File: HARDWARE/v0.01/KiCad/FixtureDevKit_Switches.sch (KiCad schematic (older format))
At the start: 58 parts, among them J10 LED_4, J11 SW_5, J12 LED_5, J13 SW_6, J14 LED_6, J15 SW_7, J2 LED_0, J3 SW_0, J4 SW_1, J5 LED_1, J6 SW_2, J7 LED_3, J8 SW_3, J9 SW_4, SW1 SW_Push_Dual, SW2 SW_Push_Dual, SW3 SW_Push_Dual, SW4 SW_Push_Dual, SW5 SW_Push_Dual, SW6 SW_Push_Dual, SW7 SW_Push_Dual, SW8 SW_Push_Dual

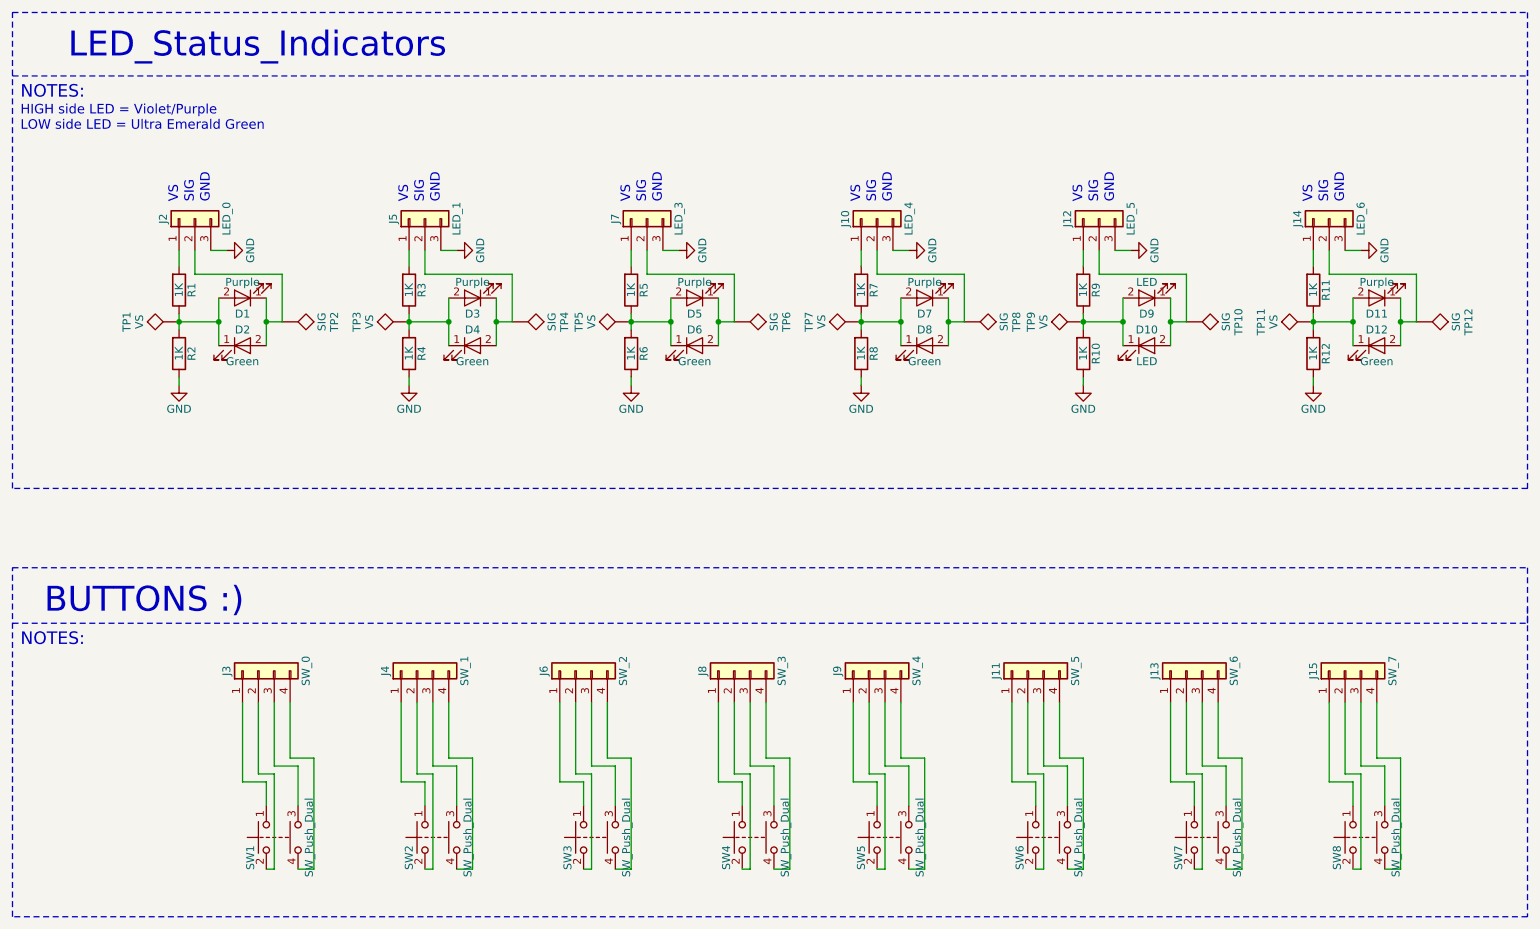
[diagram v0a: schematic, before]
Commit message: beginning pcb layout
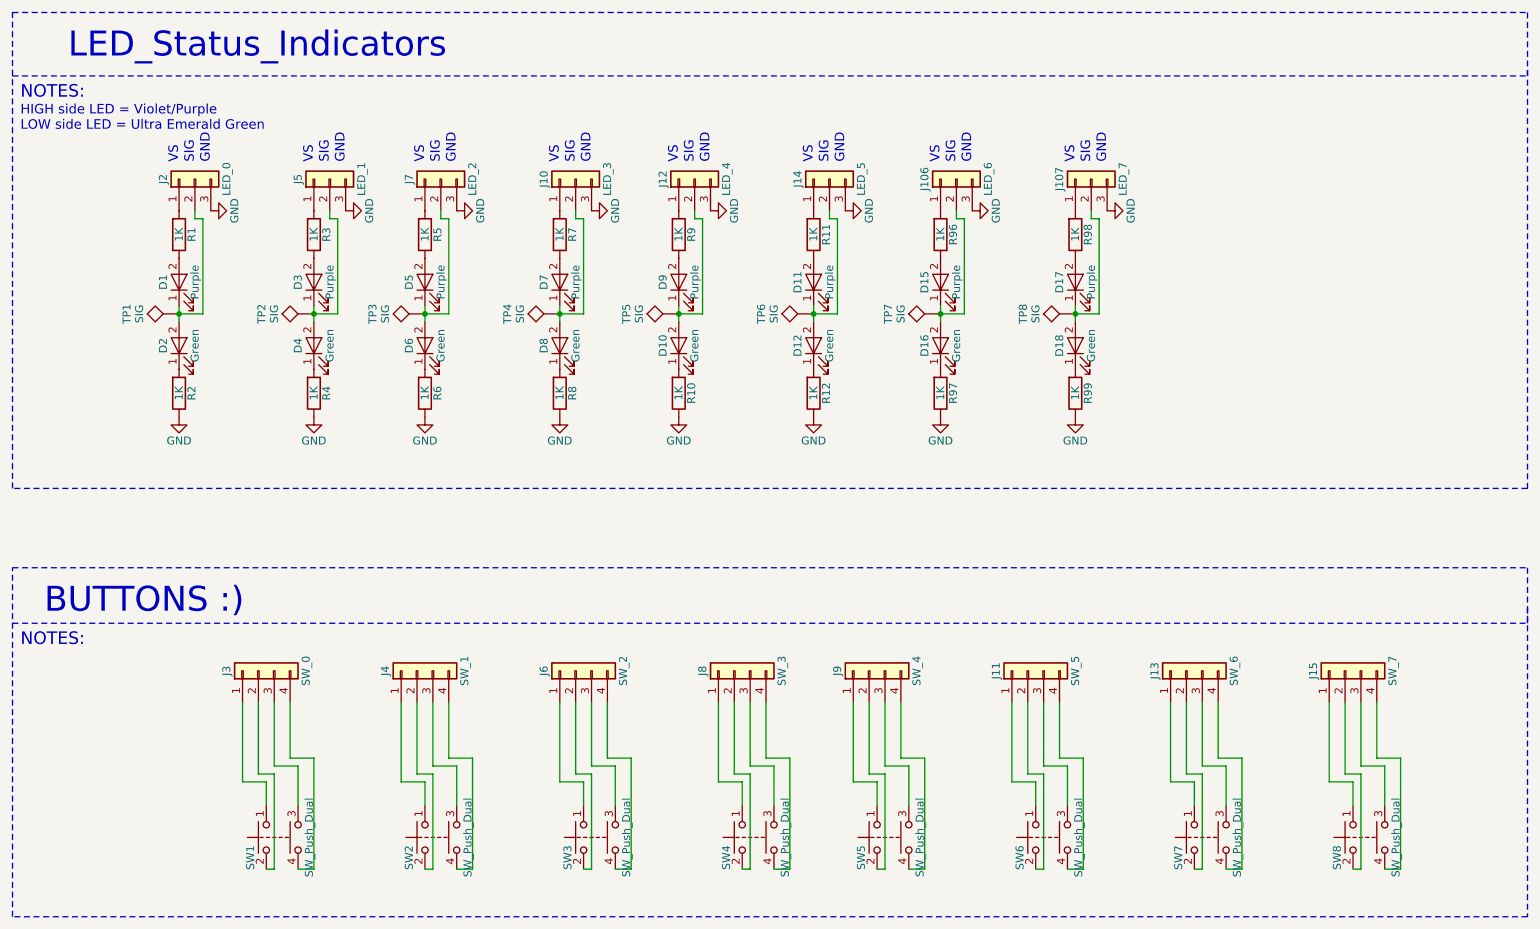
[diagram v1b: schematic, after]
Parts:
- removed TP1, TP11, TP9: VS, TestPoint:TestPoint, symbol TEST
- removed TP10, TP12: SIG, TestPoint:TestPoint, symbol TEST
- added D15, D17: Purple, LEDs:LED_0805_HandSoldering, symbol LED
- added D16, D18: Green, LEDs:LED_0805_HandSoldering, symbol LED
- added J106: LED_6, Pin_Headers:Pin_Header_Straight_1x03_Pitch2.54mm, symbol Conn_01x03
- added J107: LED_7, Pin_Headers:Pin_Header_Straight_1x03_Pitch2.54mm, symbol Conn_01x03
- added R96, R97, R98, R99: 1K, Resistors_SMD:R_0805_HandSoldering, symbol R
- added TP2: SIG, TestPoint:TestPoint, symbol TEST
- D10: value LED -> Green
- D9: value LED -> Purple
- J10: value LED_4 -> LED_3
- J12: value LED_5 -> LED_4
- J14: value LED_6 -> LED_5
- J7: value LED_3 -> LED_2
- TP3, TP5, TP7: value VS -> SIG
- renumbered TP2 to TP1
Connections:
- net GND: now also J106.3 (Pin_3), J107.3 (Pin_3), R97.1, R99.1
- net at D2.1 (K), R2.2: no longer D1.2 (A), R1.1
- net at D3.1 (K), D4.2 (A), J5.2 (Pin_2): now also TP2.1; no longer TP4.1
- net at D5.1 (K), D6.2 (A), J7.2 (Pin_2): now also TP3.1; no longer TP6.1
- net at D7.1 (K), D8.2 (A), J10.2 (Pin_2): now also TP4.1; no longer TP8.1
- net at D10.2 (A), D9.1 (K), J12.2 (Pin_2): now also TP5.1
- net at D10.1 (K), R10.2: no longer D9.2 (A), R9.1
- net at D11.1 (K), D12.2 (A), J14.2 (Pin_2): now also TP6.1
- net at D12.1 (K), R12.2: no longer D11.2 (A), R11.1
- new net: D1.2 (A), R1.1
- new net: D4.1 (K), R4.2
- new net: D3.2 (A), R3.1
- new net: D6.1 (K), R6.2
- new net: D5.2 (A), R5.1
- new net: D8.1 (K), R8.2
- new net: D7.2 (A), R7.1
- new net: D9.2 (A), R9.1
- new net: D11.2 (A), R11.1
- new net: J106.1 (Pin_1), R96.2
- new net: D15.1 (K), D16.2 (A), J106.2 (Pin_2), TP7.1
- new net: D16.1 (K), R97.2
- new net: D15.2 (A), R96.1
- new net: J107.1 (Pin_1), R98.2
- new net: D17.1 (K), D18.2 (A), J107.2 (Pin_2), TP8.1
- new net: D18.1 (K), R99.2
- new net: D17.2 (A), R98.1
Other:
- moved on the sheet: D1, D2, J2, R1, R2, TP1
